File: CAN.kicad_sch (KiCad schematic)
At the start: 5 parts, among them P1 ${MANUFACTURER PART NUMBER}, U5 ${MANUFACTURER PART NUMBER}

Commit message: rename project
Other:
- title: EPC_25 -> KA30GAN
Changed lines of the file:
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@@
   (paper "A4")
   (title_block
-    (title "EPC_25")
+    (title "KA30GAN")
     (rev "1.0")
     (company "IPM Group ©")
@@
     (pin "3")
     (instances
-      (project "EPC_25"
+      (project "ka30gan"
         (path "/2fa95553-e4bc-4555-b37d-4bed2a7cfe1b/b73927a3-d4fb-4903-bb34-b994b384e9b1"
           (reference "P1") (unit 1)
@@
     (pin "2")
     (instances
-      (project "EPC_25"
+      (project "ka30gan"
         (path "/2fa95553-e4bc-4555-b37d-4bed2a7cfe1b/b73927a3-d4fb-4903-bb34-b994b384e9b1"
           (reference "C25") (unit 1)
@@
     (pin "2")
     (instances
-      (project "EPC_25"
+      (project "ka30gan"
         (path "/2fa95553-e4bc-4555-b37d-4bed2a7cfe1b/b73927a3-d4fb-4903-bb34-b994b384e9b1"
           (reference "C24") (unit 1)
@@
     (pin "")
     (instances
-      (project "EPC_25"
+      (project "ka30gan"
         (path "/2fa95553-e4bc-4555-b37d-4bed2a7cfe1b/b73927a3-d4fb-4903-bb34-b994b384e9b1"
           (reference "#PWR040") (unit 1)
@@
     (pin "9")
     (instances
-      (project "EPC_25"
+      (project "ka30gan"
         (path "/2fa95553-e4bc-4555-b37d-4bed2a7cfe1b/b73927a3-d4fb-4903-bb34-b994b384e9b1"
           (reference "U5") (unit 1)
@@
     (pin "")
     (instances
-      (project "EPC_25"
+      (project "ka30gan"
         (path "/2fa95553-e4bc-4555-b37d-4bed2a7cfe1b/b73927a3-d4fb-4903-bb34-b994b384e9b1"
           (reference "#PWR035") (unit 1)
@@
     (pin "")
     (instances
-      (project "EPC_25"
+      (project "ka30gan"
         (path "/2fa95553-e4bc-4555-b37d-4bed2a7cfe1b/b73927a3-d4fb-4903-bb34-b994b384e9b1"
           (reference "#PWR033") (unit 1)
@@
     (pin "")
     (instances
-      (project "EPC_25"
+      (project "ka30gan"
         (path "/2fa95553-e4bc-4555-b37d-4bed2a7cfe1b/b73927a3-d4fb-4903-bb34-b994b384e9b1"
           (reference "#PWR037") (unit 1)
@@
     (pin "")
     (instances
-      (project "EPC_25"
+      (project "ka30gan"
         (path "/2fa95553-e4bc-4555-b37d-4bed2a7cfe1b/b73927a3-d4fb-4903-bb34-b994b384e9b1"
           (reference "#PWR039") (unit 1)
@@
     (pin "")
     (instances
-      (project "EPC_25"
+      (project "ka30gan"
         (path "/2fa95553-e4bc-4555-b37d-4bed2a7cfe1b/b73927a3-d4fb-4903-bb34-b994b384e9b1"
           (reference "#PWR032") (unit 1)
@@
     (pin "")
     (instances
-      (project "EPC_25"
+      (project "ka30gan"
         (path "/2fa95553-e4bc-4555-b37d-4bed2a7cfe1b/b73927a3-d4fb-4903-bb34-b994b384e9b1"
           (reference "#PWR038") (unit 1)
@@
     (pin "")
     (instances
-      (project "EPC_25"
+      (project "ka30gan"
         (path "/2fa95553-e4bc-4555-b37d-4bed2a7cfe1b/b73927a3-d4fb-4903-bb34-b994b384e9b1"
           (reference "#PWR034") (unit 1)
@@
     (pin "2")
     (instances
-      (project "EPC_25"
+      (project "ka30gan"
         (path "/2fa95553-e4bc-4555-b37d-4bed2a7cfe1b/b73927a3-d4fb-4903-bb34-b994b384e9b1"
           (reference "R15") (unit 1)
@@
     (pin "")
     (instances
-      (project "EPC_25"
+      (project "ka30gan"
         (path "/2fa95553-e4bc-4555-b37d-4bed2a7cfe1b/b73927a3-d4fb-4903-bb34-b994b384e9b1"
           (reference "#PWR036") (unit 1)

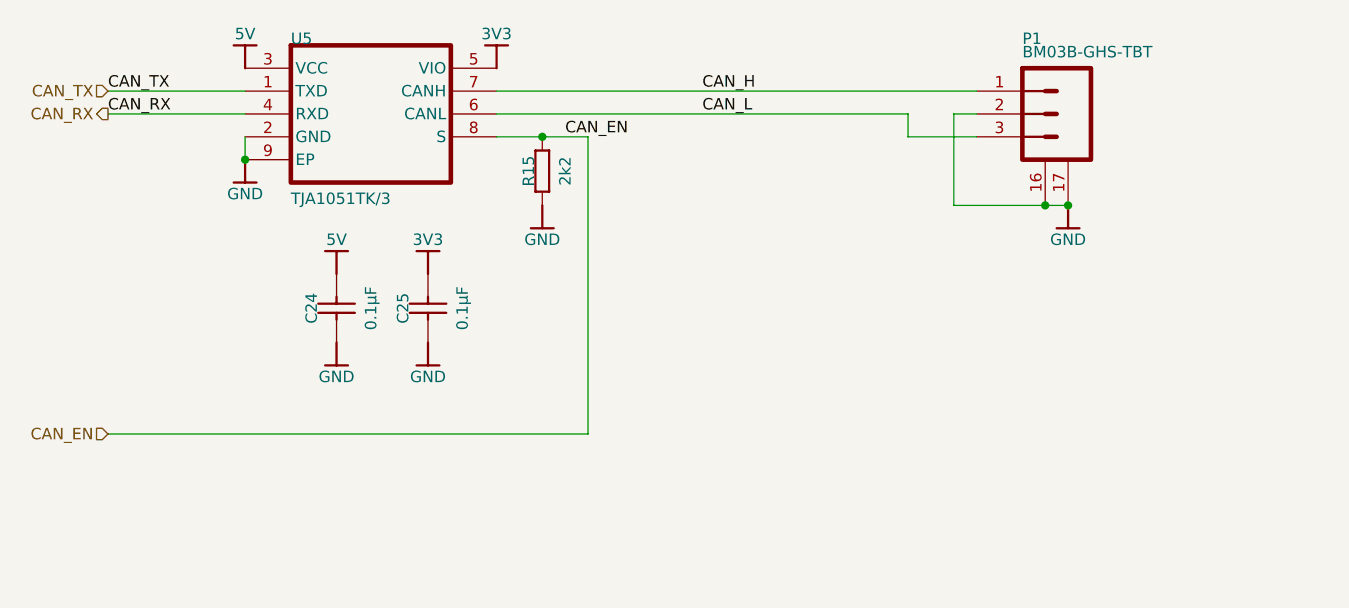
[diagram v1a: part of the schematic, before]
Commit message: edit sym
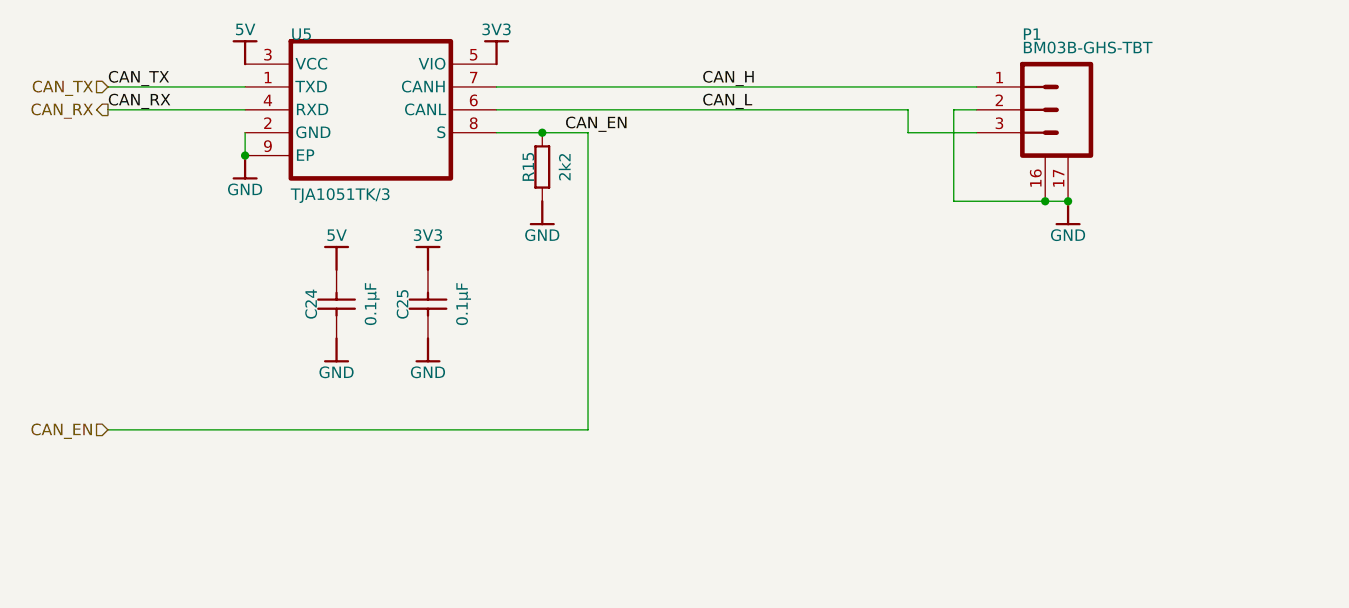
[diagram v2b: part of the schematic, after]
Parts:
- C24, C25: symbol EPC_25-altium-import:root_1_Capacitor -> ka30gan:root_1_Capacitor; ALTIUM_VALUE 0.1uF -> (none)
- P1: symbol EPC_25-altium-import:root_0_JST_GH_BM03 -> ka30gan:root_0_JST_GH_BM03; AUTHOR CERN DEM JLC -> (none)
- R15: symbol EPC_25-altium-import:root_1_Resistor -> ka30gan:root_1_Resistor; ALTIUM_VALUE 2200 -> (none)
- U5: symbol EPC_25-altium-import:root_0_TJA1051TK -> ka30gan:root_0_TJA1051TK
